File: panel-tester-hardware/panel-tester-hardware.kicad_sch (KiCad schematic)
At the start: 25 parts, among them J1 Screw_Terminal_01x02, J2 Conn_01x02, J3 Conn_01x07, Q2 BS170, U1 MCP4921, U3 LM358, U4 INA219AxD

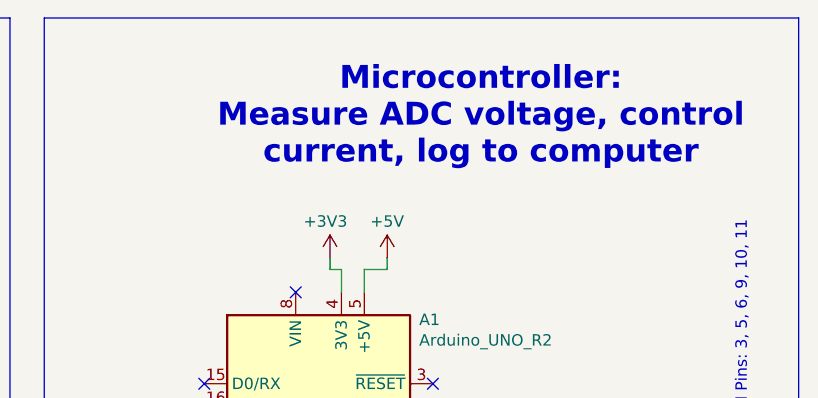
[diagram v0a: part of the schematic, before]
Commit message: Bluepill layout edits
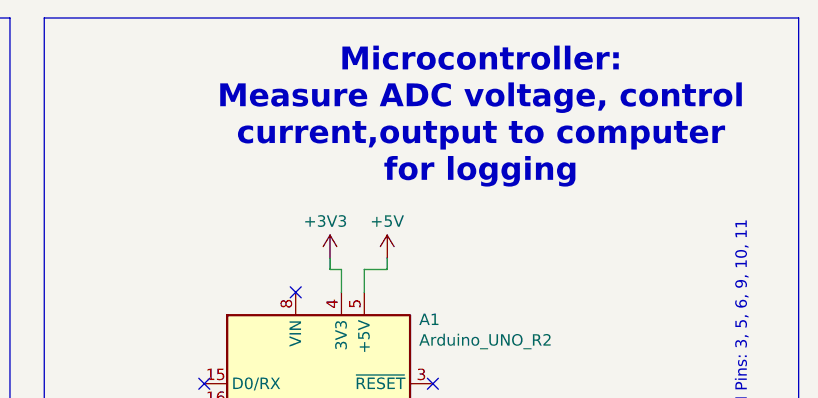
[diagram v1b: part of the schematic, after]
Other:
- note added: "Microcontroller: Measure ADC voltage, control current,output to computer for logging"
- note removed: "Microcontroller: Measure ADC voltage, control current, log to computer"
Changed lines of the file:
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@@
 	(generator_version "8.0")
 	(paper "USLetter")
+	(title_block
+		(date "2024-03-15")
+		(rev "Rev 0")
+	)
 	(junction
 		(at 105.41 83.82)
@@
 		)
 	)
-	(text "Microcontroller:\nMeasure ADC voltage, control \ncurrent, log to computer "
+	(text "Microcontroller:\nMeasure ADC voltage, control \ncurrent,output to computer \nfor logging"
 		(exclude_from_sim no)
 		(at 230.124 26.162 0)
